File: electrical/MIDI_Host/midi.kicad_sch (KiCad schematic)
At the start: 35 parts, among them U1 BL1551B, U2 BL1551B, U3 BL1551B, U4 BL1551B, U5 74HC1G14GV, U6 6N137, U7 6N137

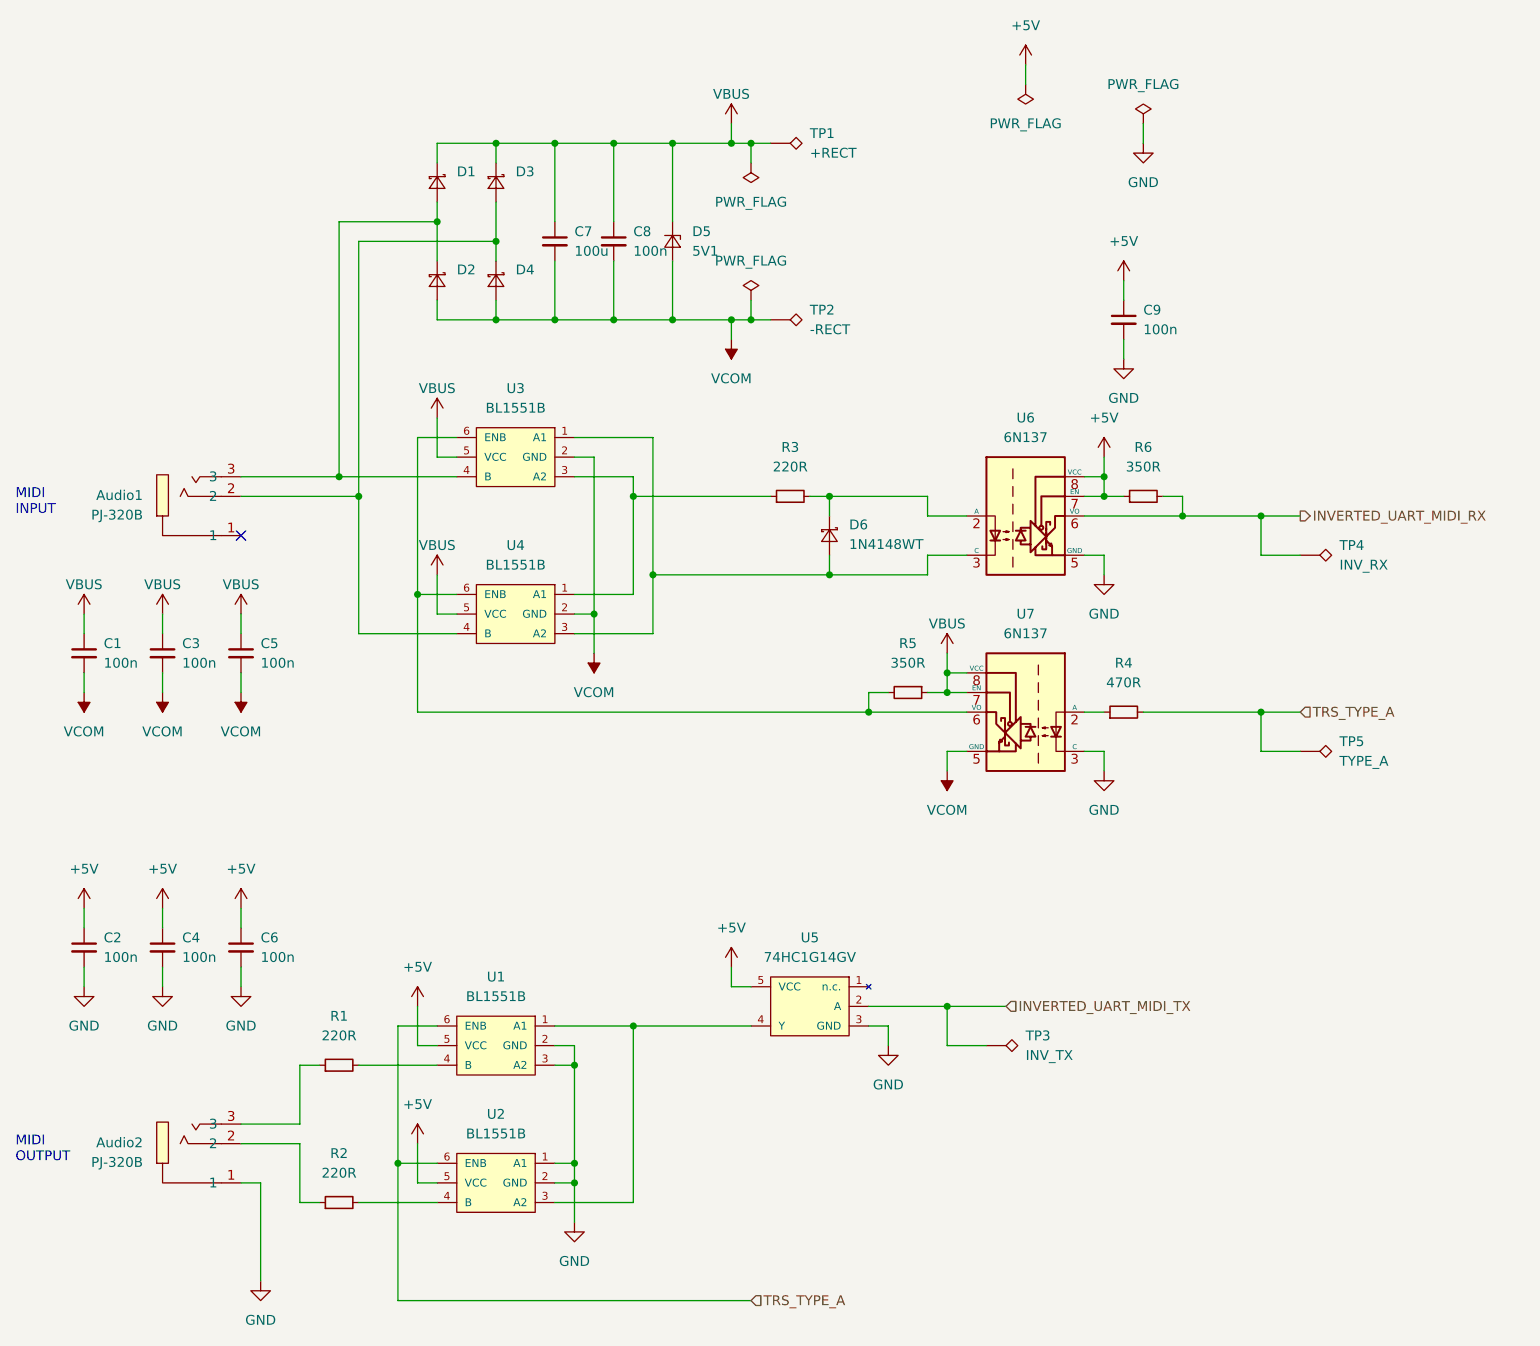
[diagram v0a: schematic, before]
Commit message: SUKU sch done
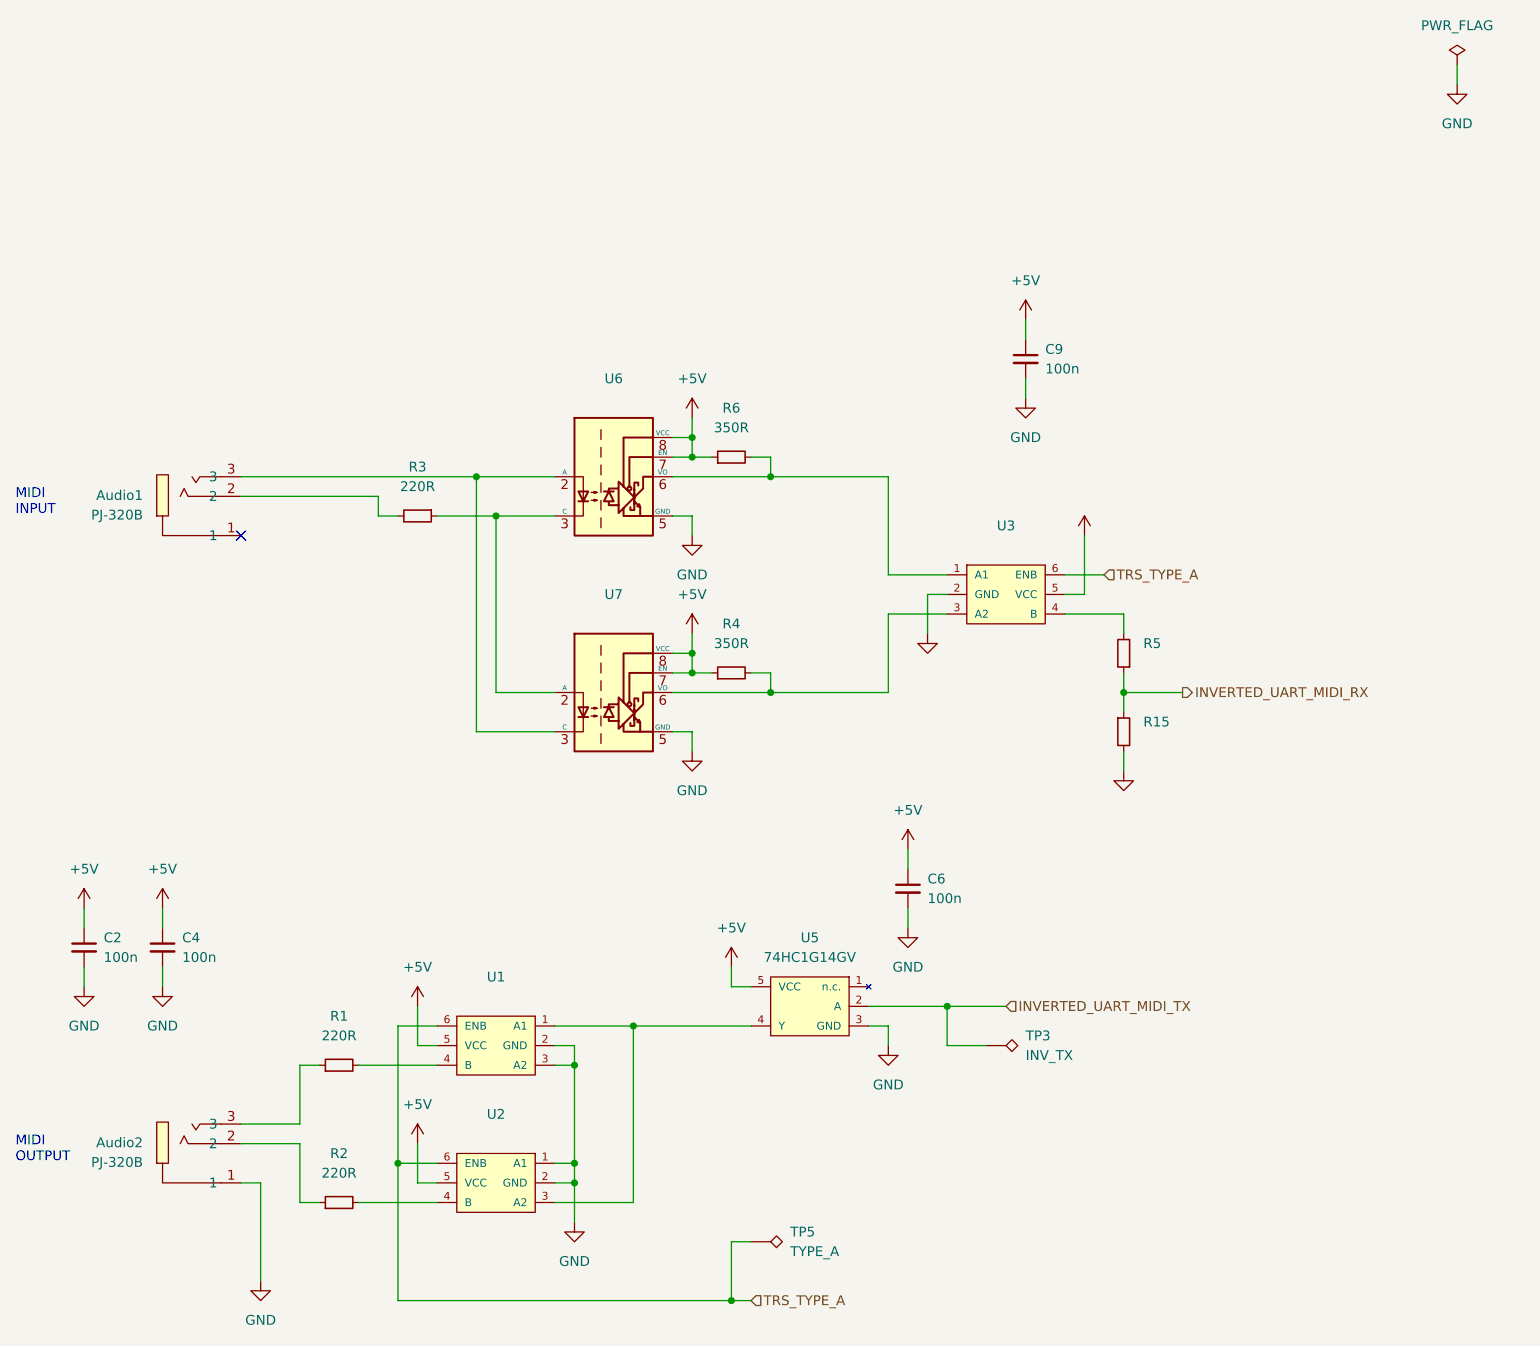
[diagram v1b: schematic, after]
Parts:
- removed C1, C3, C5, C8: 100n, suku_basics:CAP_0805, symbol suku_basics:CAP
- removed C7: 100u, suku_basics:CAP_0805, symbol suku_basics:CAP
- removed D1, D2, D3, D4, D6: 1N4148WT, Diode_SMD:D_SOD-523, symbol suku_basics:SCHOTTKY
- removed D5: 5V1, Diode_SMD:D_SOD-523, symbol suku_basics:ZENER
- removed TP1: +RECT, TestPoint:TestPoint_THTPad_1.0x1.0mm_Drill0.5mm, symbol Connector:TestPoint_Alt
- removed TP2: -RECT, TestPoint:TestPoint_THTPad_1.0x1.0mm_Drill0.5mm, symbol Connector:TestPoint_Alt
- removed TP4: INV_RX, TestPoint:TestPoint_THTPad_1.0x1.0mm_Drill0.5mm, symbol Connector:TestPoint_Alt
- removed U4: BL1551B, suku_basics:SOT-23-5-AND-TSSOP5, symbol suku_basics:BL1551B
- added R15: (no value), suku_basics:RES_0805, symbol suku_basics:RES
- R4: value 470R -> 350R
- R5: value 350R -> (none)
- U1, U2, U3: value BL1551B -> (none); footprint suku_basics:SOT-23-5-AND-TSSOP5 -> suku_basics:SOT-363_SC-70-6
- U6, U7: value 6N137 -> (none); footprint suku_basics:OPTO_SMD-8_L9.8-W6.6-P2.54-LS10.3-BL -> (none)
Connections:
- net VCOM is gone; now on net GND: U3.2 (GND), U7.5 (GND)
- net +5V: now also R4.1, U3.5 (VCC), U7.7 (EN), U7.8 (VCC)
- net GND: now also R15.2; no longer U7.3 (C)
- net INVERTED_UART_MIDI_RX: now also R5.1, R15.1; no longer R6.2, U6.6 (VO)
- net TRS_TYPE_A: now also U3.6 (ENB); no longer R4.2
- net at U6.2 (A): now also Audio1.3, U7.3 (C); no longer R3.2
- net at U6.3 (C): now also R3.1, U7.2 (A); no longer U3.1 (A1)
- net at Audio1.2: now also R3.2
- net at U3.4 (B): now also R5.2; no longer Audio1.3
- net at U3.3 (A2): now also R4.2, U7.6 (VO); no longer R3.1
- removed net VBUS: R5.1, U3.5 (VCC), U7.7 (EN), U7.8 (VCC)
- new net: R6.2, U3.1 (A1), U6.6 (VO)
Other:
- moved on the sheet: C6, C9, R3, R6, TP5, U6, U7
